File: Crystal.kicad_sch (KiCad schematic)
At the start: 3 parts

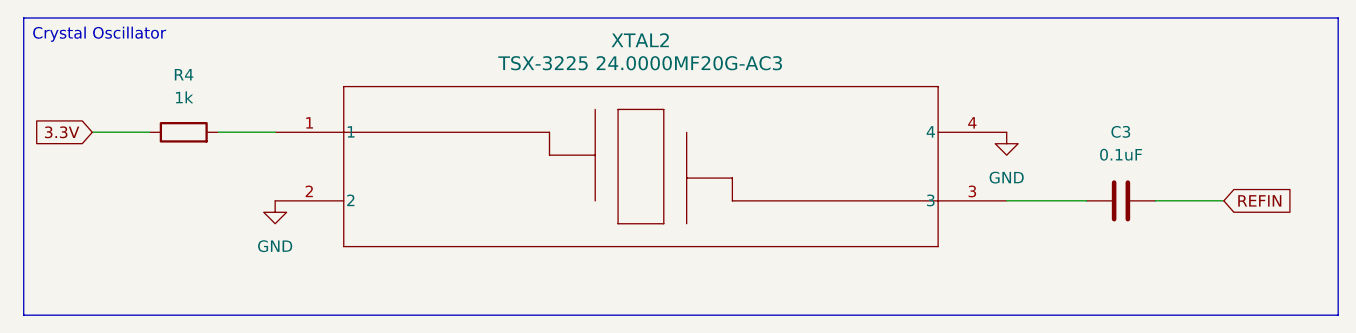
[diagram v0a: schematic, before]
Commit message: updated schematic
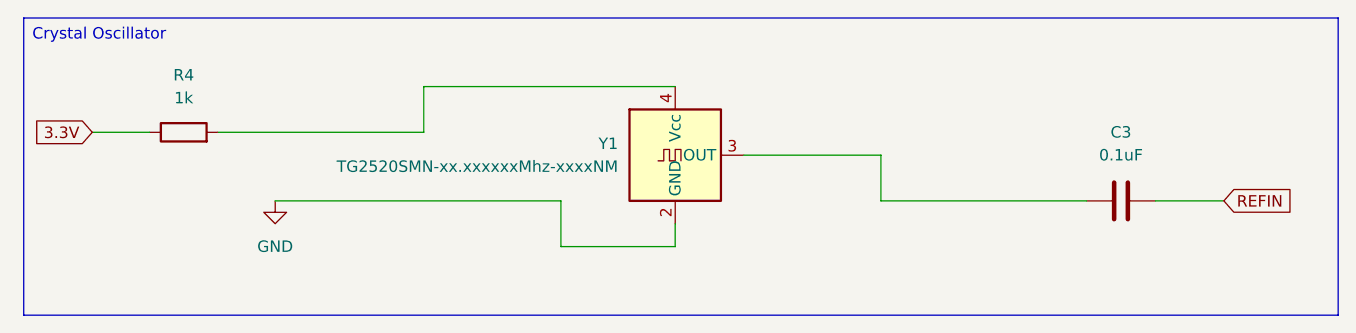
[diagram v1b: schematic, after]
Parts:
- removed XTAL2: TSX-3225 24.0000MF20G-AC3, TSX-3225 24.0000MF20G-AC3_EPS, symbol TSX_3225_24_0000MF20G_AC3:TSX-3225_24.0000MF20G-AC3
- added Y1: TG2520SMN-xx.xxxxxxMhz-xxxxNM, Oscillator:Oscillator_SMD_SeikoEpson_TG2520SMN-xxx-xxxxxx-4Pin_2.5x2.0mm, symbol Oscillator:TG2520SMN-xx.xxxxxxMhz-xxxxNM
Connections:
- net GND: now also Y1.2 (GND)
- net at R4.2: now also Y1.4 (Vcc)
- net at C3.2: now also Y1.3 (OUT)
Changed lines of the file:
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@@
+	(wire
+		(pts
+			(xy 132.08 102.87) (xy 144.78 102.87)
+		)
+		(stroke
+			(width 0)
+			(type default)
+		)
+	)
 	(wire
 		(pts
@@
 	(wire
 		(pts
-			(xy 93.98 90.17) (xy 100.33 90.17)
+			(xy 152.4 92.71) (xy 167.64 92.71)
+		)
+		(stroke
+			(width 0)
+			(type default)
+		)
+	)
+	(wire
+		(pts
+			(xy 116.84 90.17) (xy 116.84 85.09)
+		)
+		(stroke
+			(width 0)
+			(type default)
+		)
+	)
+	(wire
+		(pts
+			(xy 93.98 90.17) (xy 116.84 90.17)
 		)
 		(stroke
@@
 	(wire
 		(pts
-			(xy 181.61 97.79) (xy 190.5 97.79)
+			(xy 144.78 102.87) (xy 144.78 100.33)
+		)
+		(stroke
+			(width 0)
+			(type default)
+		)
+	)
+	(wire
+		(pts
+			(xy 167.64 97.79) (xy 190.5 97.79)
+		)
+		(stroke
+			(width 0)
+			(type default)
+		)
+	)
+	(wire
+		(pts
+			(xy 100.33 97.79) (xy 132.08 97.79)
+		)
+		(stroke
+			(width 0)
+			(type default)
+		)
+	)
+	(wire
+		(pts
+			(xy 132.08 97.79) (xy 132.08 102.87)
+		)
+		(stroke
+			(width 0)
+			(type default)
+		)
+	)
+	(wire
+		(pts
+			(xy 116.84 85.09) (xy 144.78 85.09)
+		)
+		(stroke
+			(width 0)
+			(type default)
+		)
+	)
+	(wire
+		(pts
+			(xy 167.64 92.71) (xy 167.64 97.79)
 		)
 		(stroke
@@
 	)
 	(symbol
-		(lib_id "TSX_3225_24_0000MF20G_AC3:TSX-3225_24.0000MF20G-AC3")
-		(at 100.33 92.71 0)
+		(lib_id "Oscillator:TG2520SMN-xx.xxxxxxMhz-xxxxNM")
+		(at 144.78 92.71 0)
 		(unit 1)
 		(exclude_from_sim no)
@@
 		(dnp no)
 		(fields_autoplaced yes)
-		(property "Reference" "XTAL2"
-			(at 140.97 80.01 0)
-			(effects
-				(font
-					(size 1.524 1.524)
-				)
-			)
-		)
-		(property "Value" "TSX-3225 24.0000MF20G-AC3"
-			(at 140.97 82.55 0)
-			(effects
-				(font
-					(size 1.524 1.524)
-				)
-			)
-		)
-		(property "Footprint" "TSX-3225 24.0000MF20G-AC3_EPS"
-			(at 100.33 92.71 0)
-			(effects
-				(font
-					(size 1.27 1.27)
-					(italic yes)
-				)
-				(hide yes)
-			)
-		)
-		(property "Datasheet" "TSX-3225 24.0000MF20G-AC3"
-			(at 100.33 92.71 0)
-			(effects
-				(font
-					(size 1.27 1.27)
-					(italic yes)
-				)
-				(hide yes)
-			)
-		)
-		(property "Description" ""
-			(at 100.33 92.71 0)
-			(effects
-				(font
-					(size 1.27 1.27)
-				)
-				(hide yes)
-			)
+		(property "Reference" "Y1"
+			(at 138.43 91.4399 0)
+			(effects
+				(font
+					(size 1.27 1.27)
+				)
+				(justify right)
+			)
+		)
+		(property "Value" "TG2520SMN-xx.xxxxxxMhz-xxxxNM"
+			(at 138.43 93.9799 0)
+			(effects
+				(font
+					(size 1.27 1.27)
+				)
+				(justify right)
+			)
+		)
+		(property "Footprint" "Oscillator:Oscillator_SMD_SeikoEpson_TG2520SMN-xxx-xxxxxx-4Pin_2.5x2.0mm"
+			(at 156.21 101.6 0)
+			(effects
+				(font
+					(size 1.27 1.27)
+				)
+				(hide yes)
+			)
+		)
+		(property "Datasheet" "https://support.epson.biz/td/api/doc_check.php?dl=app_TG2520SMN&lang=en"
+			(at 142.24 92.71 0)
+			(effects
+				(font
+					(size 1.27 1.27)
+				)
+				(hide yes)
+			)
+		)
+		(property "Description" "Crystal Oscillator Low Profile / High Stability TCXO"
+			(at 144.78 92.71 0)
+			(effects
+				(font
+					(size 1.27 1.27)
+				)
+				(hide yes)
+			)
+		)
+		(pin "4"
+		)
+		(pin "1"
+		)
+		(pin "2"
 		)
 		(pin "3"
 		)
-		(pin "4"
-		)
-		(pin "1"
-		)
-		(pin "2"
-		)
 		(instances
-			(project "RFclockgen"
+			(project ""
 				(path "/e1444a2d-a0c4-493c-a136-c624dc084e46/e0719063-0868-4156-844d-b05e9bfe86b9"
-					(reference "XTAL2")
+					(reference "Y1")
 					(unit 1)
 				)
-			)
-		)
-	)
-	(symbol
-		(lib_id "power:GND")
-		(at 181.61 90.17 0)
-		(unit 1)
-		(exclude_from_sim no)
-		(in_bom yes)
-		(on_board yes)
-		(dnp no)
-		(fields_autoplaced yes)
-		(property "Reference" "#PWR07"
-			(at 181.61 96.52 0)
-			(effects
-				(font
-					(size 1.27 1.27)
-				)
-				(hide yes)
-			)
-		)
-		(property "Value" "GND"
-			(at 181.61 95.25 0)
-			(effects
-				(font
-					(size 1.27 1.27)
-				)
-			)
-		)
-		(property "Footprint" ""
-			(at 181.61 90.17 0)
-			(effects
-				(font
-					(size 1.27 1.27)
-				)
-				(hide yes)
-			)
-		)
-		(property "Datasheet" ""
-			(at 181.61 90.17 0)
-			(effects
-				(font
-					(size 1.27 1.27)
-				)
-				(hide yes)
-			)
-		)
-		(property "Description" "Power symbol creates a global label with name \"GND\" , ground"
-			(at 181.61 90.17 0)
-			(effects
-				(font
-					(size 1.27 1.27)
-				)
-				(hide yes)
-			)
-		)
-		(pin "1"
-		)
-		(instances
-			(project "RFclockgen"
-				(path "/e1444a2d-a0c4-493c-a136-c624dc084e46/e0719063-0868-4156-844d-b05e9bfe86b9"
-					(reference "#PWR07")
-					(unit 1)
-				)
